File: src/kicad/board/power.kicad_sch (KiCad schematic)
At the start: 16 parts, among them Q1 DMG2301L, U3 XB8089D, U4 BQ24090DGQ

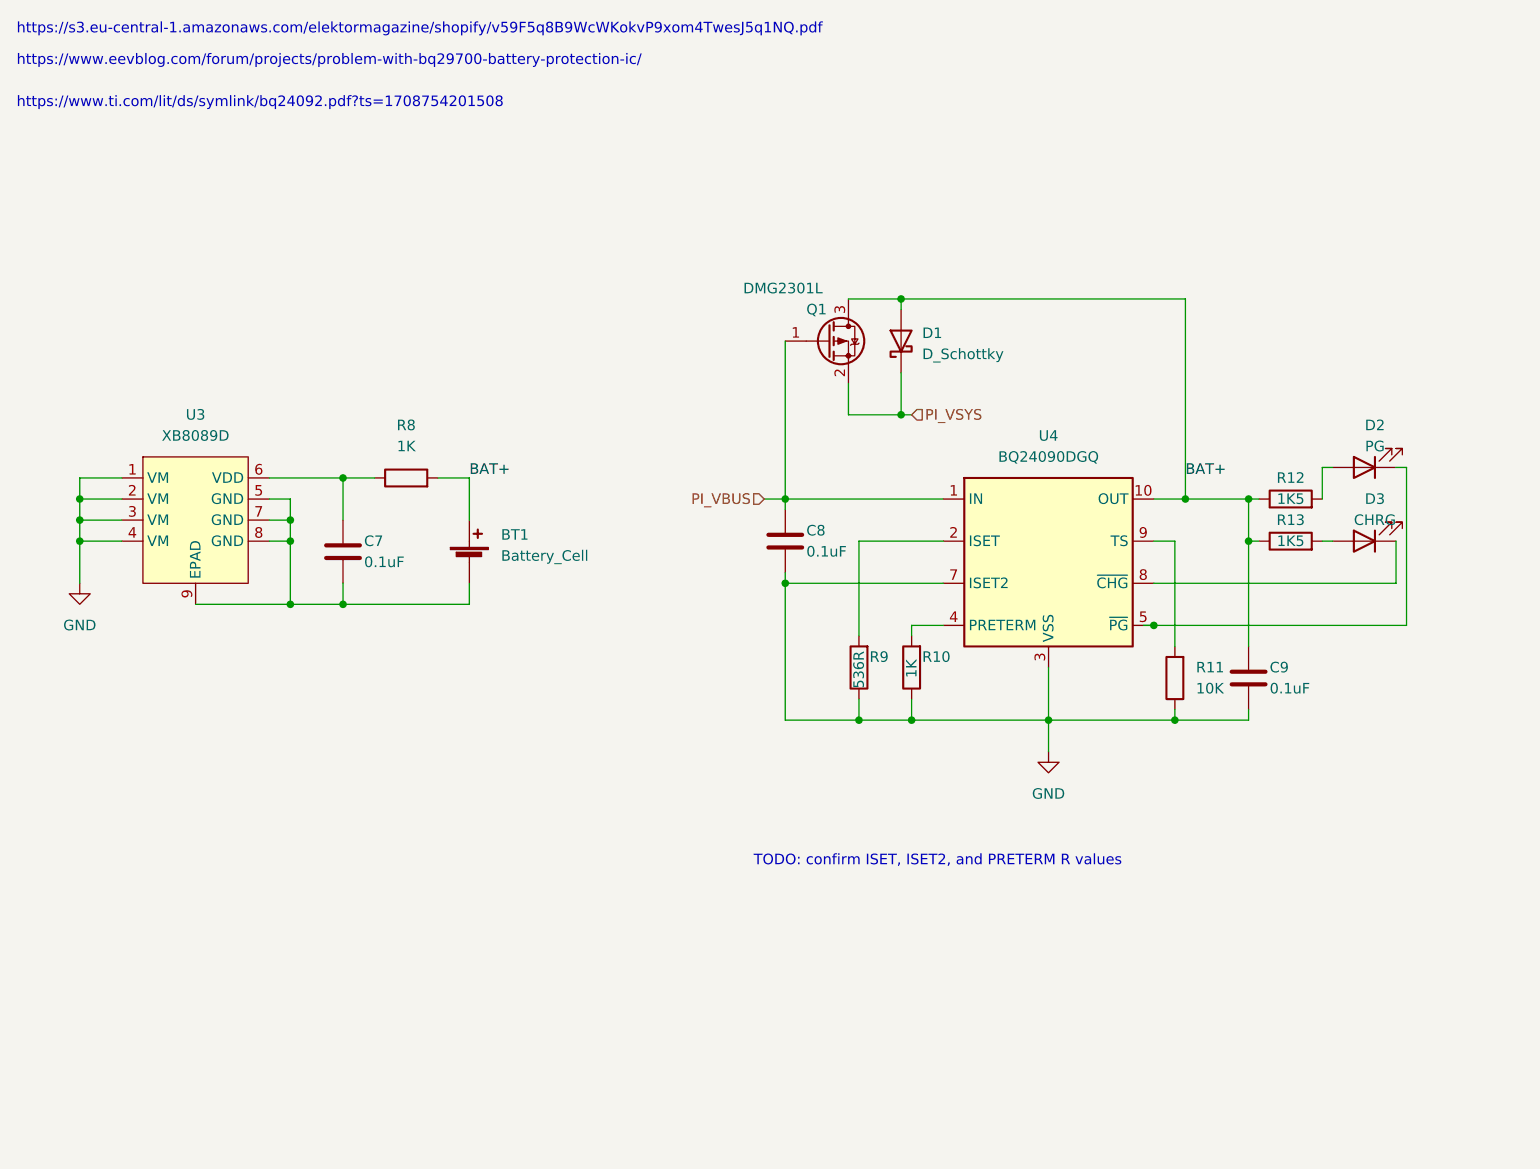
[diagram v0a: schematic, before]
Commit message: cleanup
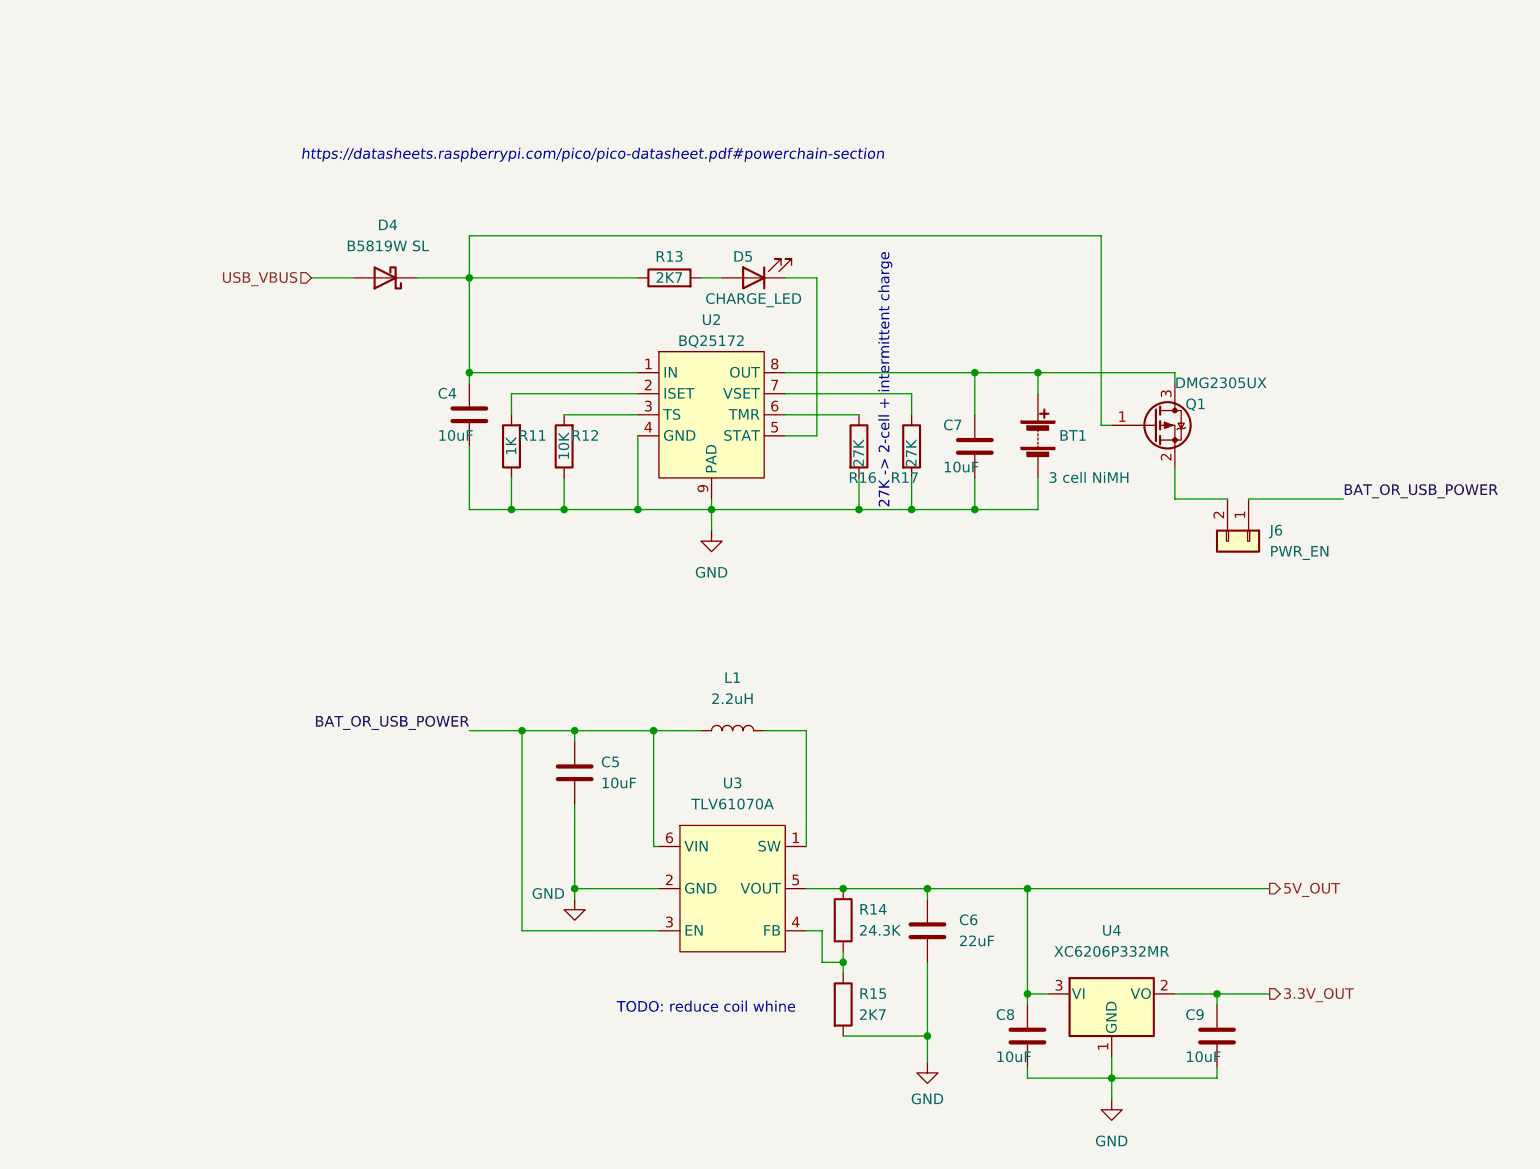
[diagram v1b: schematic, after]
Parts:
- removed BT1: Battery_Cell, symbol Device:Battery_Cell
- removed D1: D_Schottky, symbol Device:D_Schottky
- removed D2: PG, symbol Device:LED
- removed D3: CHRG, symbol Device:LED
- removed R10, R8: 1K, symbol Device:R
- removed R9: 536R, symbol Device:R
- removed U3: XB8089D, Library:XB8089D, symbol project_library:XB8089D
- removed U4: BQ24090DGQ, Package_SO:HVSSOP-10-1EP_3x3mm_P0.5mm_EP1.57x1.88mm_ThermalVias, symbol Battery_Management:BQ24090DGQ
- added BT1: 3 cell NiMH, Battery:BatteryHolder_Keystone_2462_2xAA, symbol Device:Battery
- added C4, C5: 10uF, Capacitor_SMD:C_0603_1608Metric, symbol Device:C
- added C6: 22uF, Capacitor_SMD:C_0603_1608Metric, symbol Device:C
- added D4: B5819W SL, Diode_SMD:D_SOD-123, symbol Diode:1N5819
- added D5: CHARGE_LED, LED_SMD:LED_0805_2012Metric, symbol Device:LED
- added J6: PWR_EN, Connector_PinHeader_2.54mm:PinHeader_1x02_P2.54mm_Vertical, symbol Connector_Generic:Conn_01x02
- added L1: 2.2uH, Inductor_SMD:L_Sunlord_MWSA05xxS, symbol Device:L
- added R14: 24.3K, Resistor_SMD:R_0805_2012Metric, symbol Device:R
- added R15: 2K7, Resistor_SMD:R_0603_1608Metric, symbol Device:R
- added R16, R17: 27K, Resistor_SMD:R_0603_1608Metric, symbol Device:R
- added U2: BQ25172, Package_SON:WSON-8-1EP_2x2mm_P0.5mm_EP0.9x1.6mm, symbol project_library:BQ25172
- added U3: TLV61070A, Package_SO:TSOP-6_1.65x3.05mm_P0.95mm, symbol project_library:TLV61070A
- added U4: XC6206P332MR, Package_TO_SOT_SMD:SOT-23-3, symbol Regulator_Linear:XC6206PxxxMR
- C7, C8, C9: value 0.1uF -> 10uF; footprint (none) -> Capacitor_SMD:C_0603_1608Metric; Vendor (none) -> C19702
- Q1: value DMG2301L -> DMG2305UX; Vendor (none) -> C2940629
- R11: value 10K -> 1K; footprint (none) -> Resistor_SMD:R_0603_1608Metric; Vendor (none) -> C21190
- R12: value 1K5 -> 10K; footprint (none) -> Resistor_SMD:R_0603_1608Metric; Vendor (none) -> C25804
- R13: value 1K5 -> 2K7; footprint (none) -> Resistor_SMD:R_0603_1608Metric; Vendor (none) -> C13167
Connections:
- net GND: now also C7.2, R12.1, BT1.2 (-), C4.2, C5.2, C6.2, R15.2, R16.2, R17.2, U2.4 (GND), U2.9 (PAD), U3.2 (GND), U4.1 (GND)
- net at R13.2: now also D5.2 (A)
- net at C7.1: now also Q1.3 (D), BT1.1 (+), U2.8 (OUT)
- net at R11.2: now also U2.2 (ISET)
- net at R12.2: now also U2.3 (TS)
- removed net BAT+: C9.1, Q1.3 (D), R12.1, R13.1
- net PI_VBUS: no longer names the net of Q1.1 (G)
- net PI_VBUS: now also R13.1, C4.1, D4.1 (K), U2.1 (IN); no longer C8.1
- net PI_VSYS: no longer names the net of Q1.2 (S)
- net PI_VSYS: now also J6.2 (Pin_2)
- new net: R17.1, U2.7 (VSET)
- new net: R14.2, R15.1, U3.4 (FB)
- new net: D5.1 (K), U2.5 (STAT)
- new net: L1.2, U3.1 (SW)
- new net: R16.1, U2.6 (TMR)
- new net 3.3V_OUT: C9.1, U4.2 (VO)
- new net 5V_OUT: C6.1, C8.1, R14.1, U3.5 (VOUT), U4.3 (VI)
- new net BAT_OR_USB_POWER: C5.1, J6.1 (Pin_1), L1.1, U3.3 (EN), U3.6 (VIN)
- new net USB_VBUS: D4.2 (A)
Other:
- note added: "27K -> 2-cell + intermittent charge"
- note added: "TODO: reduce coil whine"
- note added: "https://datasheets.raspberrypi.com/pico/pico-datasheet.pdf#powerchain-section"
- note removed: "TODO: confirm ISET, ISET2, and PRETERM R values"
- note removed: "https://s3.eu-central-1.amazonaws.com/elektormagazine/shopify/v59F5q8B9WcWKokvP9xom4TwesJ5q1NQ.pdf"
- note removed: "https://www.eevblog.com/forum/projects/problem-with-bq29700-battery-protection-ic/"
- note removed: "https://www.ti.com/lit/ds/symlink/bq24092.pdf?ts=1708754201508"
